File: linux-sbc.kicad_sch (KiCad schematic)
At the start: 9 parts, among them J101 Molex Mini-fit Jr

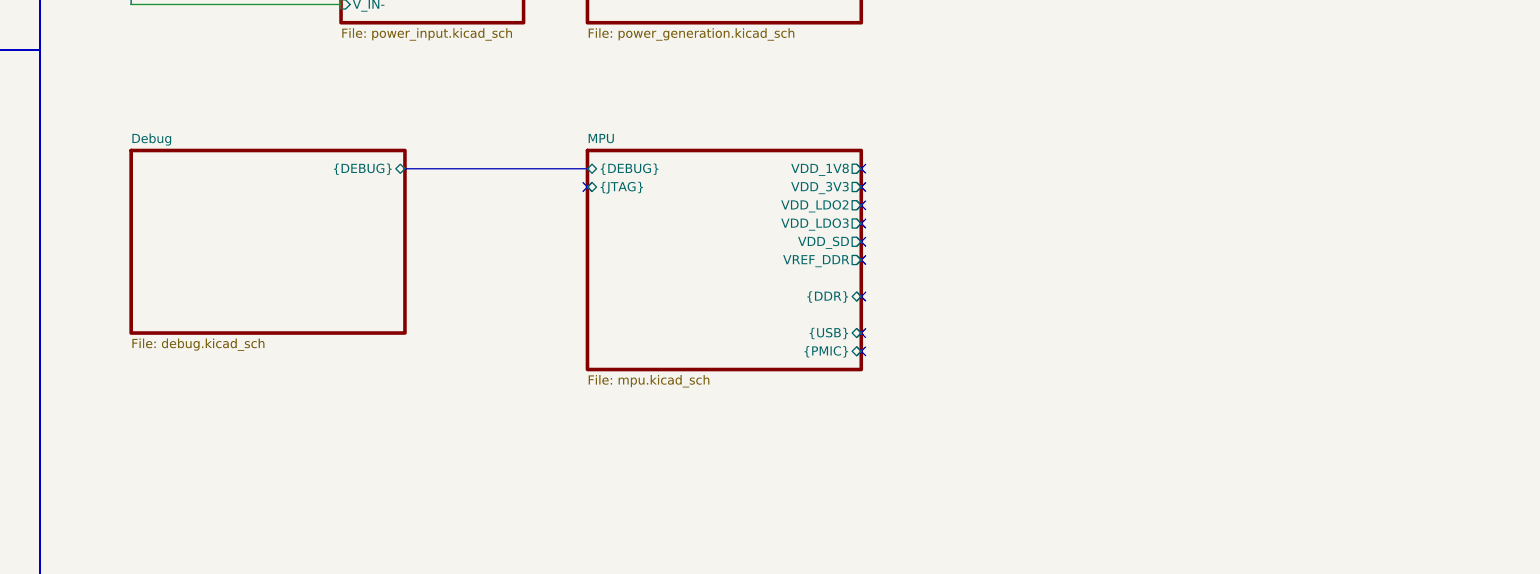
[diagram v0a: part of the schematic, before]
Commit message: Add a debug section
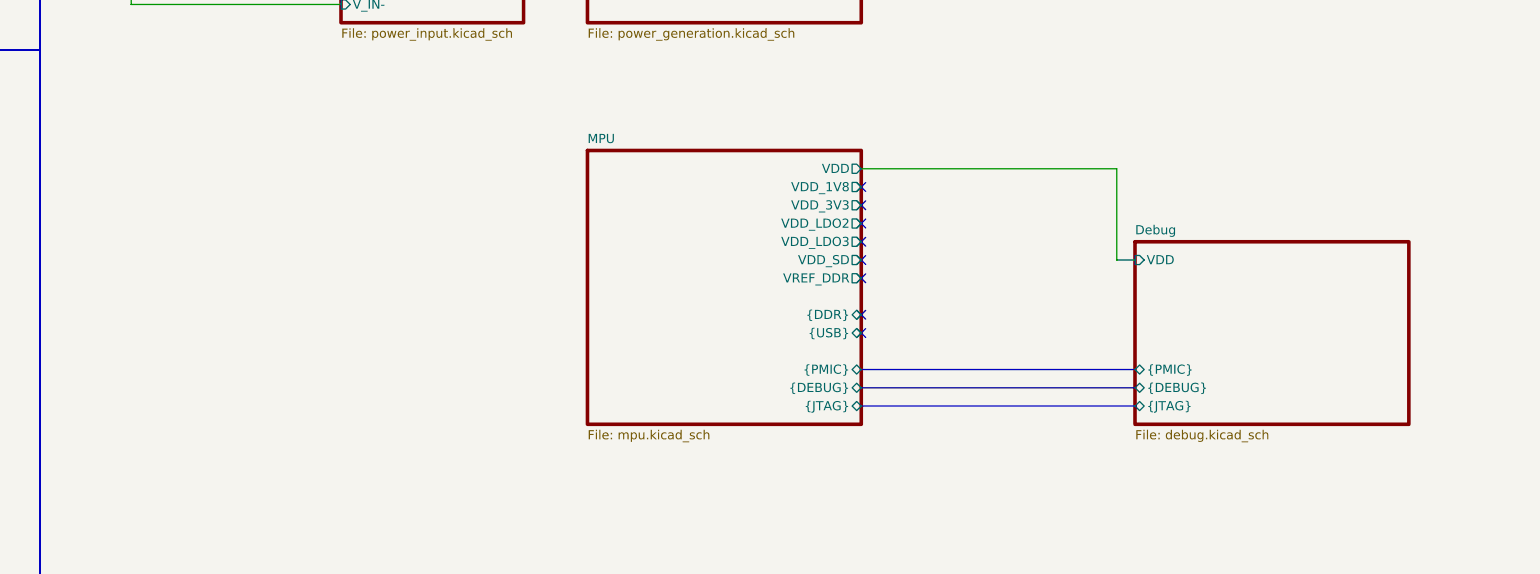
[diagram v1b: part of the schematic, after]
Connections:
- no-connect marks 10 -> 8
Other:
- sheet Debug ports: added VDD, {JTAG}, {PMIC}; removed none
- sheet MPU ports: added VDD; removed none
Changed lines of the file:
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@@
 			)
 			(justify left)
-			(href "#3")
+			(href "#4")
 		)
 	)
@@
 			)
 			(justify left)
-			(href "#3")
+			(href "#7")
 		)
 	)
@@
 			)
 			(justify left)
-			(href "#4")
+			(href "#6")
 		)
 	)
@@
 			)
 			(justify left)
-			(href "#4")
+			(href "#5")
 		)
 	)
@@
 	)
 	(no_connect
+		(at 254 139.7)
+	)
+	(no_connect
+		(at 254 144.78)
+	)
+	(no_connect
 		(at 254 137.16)
 	)
 	(no_connect
-		(at 215.9 132.08)
+		(at 254 149.86)
+	)
+	(no_connect
+		(at 254 132.08)
 	)
 	(no_connect
@@
 	)
 	(no_connect
+		(at 254 152.4)
+	)
+	(no_connect
 		(at 254 134.62)
 	)
-	(no_connect
-		(at 254 147.32)
-	)
-	(no_connect
-		(at 254 129.54)
-	)
-	(no_connect
-		(at 254 139.7)
-	)
-	(no_connect
-		(at 254 154.94)
-	)
-	(no_connect
-		(at 254 152.4)
-	)
-	(no_connect
-		(at 254 132.08)
-	)
 	(wire
 		(pts
@@
 		)
 	)
+	(bus
+		(pts
+			(xy 254 162.56) (xy 292.1 162.56)
+		)
+		(stroke
+			(width 0)
+			(type default)
+		)
+	)
 	(wire
 		(pts
@@
 	(wire
 		(pts
+			(xy 289.56 142.24) (xy 292.1 142.24)
+		)
+		(stroke
+			(width 0)
+			(type default)
+		)
+	)
+	(wire
+		(pts
 			(xy 167.64 88.9) (xy 167.64 91.44)
 		)
@@
 	(wire
 		(pts
+			(xy 289.56 129.54) (xy 289.56 142.24)
+		)
+		(stroke
+			(width 0)
+			(type default)
+		)
+	)
+	(wire
+		(pts
 			(xy 166.37 88.9) (xy 167.64 88.9)
 		)
@@
 		)
 	)
+	(bus
+		(pts
+			(xy 254 160.02) (xy 292.1 160.02)
+		)
+		(stroke
+			(width 0)
+			(type default)
+		)
+	)
+	(bus
+		(pts
+			(xy 254 157.48) (xy 292.1 157.48)
+		)
+		(stroke
+			(width 0)
+			(type default)
+		)
+	)
 	(wire
 		(pts
@@
 		)
 	)
-	(bus
-		(pts
-			(xy 190.5 129.54) (xy 215.9 129.54)
+	(wire
+		(pts
+			(xy 254 129.54) (xy 289.56 129.54)
 		)
 		(stroke
@@
 	(sheet
 		(at 215.9 127)
-		(size 38.1 30.48)
+		(size 38.1 38.1)
 		(exclude_from_sim no)
 		(in_bom yes)
@@
 		)
 		(property "Sheetfile" "mpu.kicad_sch"
-			(at 215.9 158.2384 0)
+			(at 215.9 165.8584 0)
 			(effects
 				(font
@@
 		)
 		(pin "{DDR}" bidirectional
-			(at 254 147.32 0)
+			(at 254 149.86 0)
 			(effects
 				(font
@@
 		)
 		(pin "{JTAG}" bidirectional
-			(at 215.9 132.08 180)
-			(effects
-				(font
-					(size 1.27 1.27)
-				)
-				(justify left)
+			(at 254 162.56 0)
+			(effects
+				(font
+					(size 1.27 1.27)
+				)
+				(justify right)
 			)
 		)
@@
 		)
 		(pin "VDD_1V8" output
+			(at 254 132.08 0)
+			(effects
+				(font
+					(size 1.27 1.27)
+				)
+				(justify right)
+			)
+		)
+		(pin "VDD_3V3" output
+			(at 254 134.62 0)
+			(effects
+				(font
+					(size 1.27 1.27)
+				)
+				(justify right)
+			)
+		)
+		(pin "VDD_LDO2" output
+			(at 254 137.16 0)
+			(effects
+				(font
+					(size 1.27 1.27)
+				)
+				(justify right)
+			)
+		)
+		(pin "VDD_LDO3" output
+			(at 254 139.7 0)
+			(effects
+				(font
+					(size 1.27 1.27)
+				)
+				(justify right)
+			)
+		)
+		(pin "VDD_SD" output
+			(at 254 142.24 0)
+			(effects
+				(font
+					(size 1.27 1.27)
+				)
+				(justify right)
+			)
+		)
+		(pin "VREF_DDR" output
+			(at 254 144.78 0)
+			(effects
+				(font
+					(size 1.27 1.27)
+				)
+				(justify right)
+			)
+		)
+		(pin "{PMIC}" bidirectional
+			(at 254 157.48 0)
+			(effects
+				(font
+					(size 1.27 1.27)
+				)
+				(justify right)
+			)
+		)
+		(pin "{DEBUG}" bidirectional
+			(at 254 160.02 0)
+			(effects
+				(font
+					(size 1.27 1.27)
+				)
+				(justify right)
+			)
+		)
+		(pin "VDD" output
 			(at 254 129.54 0)
 			(effects
@@
 				)
 				(justify right)
-			)
-		)
-		(pin "VDD_3V3" output
-			(at 254 132.08 0)
-			(effects
-				(font
-					(size 1.27 1.27)
-				)
-				(justify right)
-			)
-		)
-		(pin "VDD_LDO2" output
-			(at 254 134.62 0)
-			(effects
-				(font
-					(size 1.27 1.27)
-				)
-				(justify right)
-			)
-		)
-		(pin "VDD_LDO3" output
-			(at 254 137.16 0)
-			(effects
-				(font
-					(size 1.27 1.27)
-				)
-				(justify right)
-			)
-		)
-		(pin "VDD_SD" output
-			(at 254 139.7 0)
-			(effects
-				(font
-					(size 1.27 1.27)
-				)
-				(justify right)
-			)
-		)
-		(pin "VREF_DDR" output
-			(at 254 142.24 0)
-			(effects
-				(font
-					(size 1.27 1.27)
-				)
-				(justify right)
-			)
-		)
-		(pin "{PMIC}" bidirectional
-			(at 254 154.94 0)
-			(effects
-				(font
-					(size 1.27 1.27)
-				)
-				(justify right)
-			)
-		)
-		(pin "{DEBUG}" bidirectional
-			(at 215.9 129.54 180)
-			(effects
-				(font
-					(size 1.27 1.27)
-				)
-				(justify left)
 			)
 		)
@@
 	)
 	(sheet
-		(at 152.4 127)
+		(at 292.1 139.7)
 		(size 38.1 25.4)
 		(exclude_from_sim no)
@@
 		)
 		(property "Sheetname" "Debug"
-			(at 152.4 126.1146 0)
+			(at 292.1 138.8146 0)
 			(effects
 				(font
@@
 		)
 		(property "Sheetfile" "debug.kicad_sch"
-			(at 152.4 153.1584 0)
+			(at 292.1 165.8584 0)
 			(effects
 				(font
@@
 		)
 		(pin "{DEBUG}" bidirectional
-			(at 190.5 129.54 0)
-			(effects
-				(font
-					(size 1.27 1.27)
-				)
-				(justify right)
-			)
-		)
+			(at 292.1 160.02 180)
+			(effects
+				(font
+					(size 1.27 1.27)
+				)
+				(justify left)
+			)
+		)
+		(pin "VDD" input
+			(at 292.1 142.24 180)
+			(effects
+				(font
+					(size 1.27 1.27)
+				)
+				(justify left)
+			)
+		)
+		(pin "{JTAG}" bidirectional
+			(at 292.1 162.56 180)
+			(effects
+				(font
+					(size 1.27 1.27)
+				)
+				(justify left)
+			)
+		)
+		(pin "{PMIC}" bidirectional
+			(at 292.1 157.48 180)
+			(effects
+				(font
+					(size 1.27 1.27)
+				)
+				(justify left)
+			)
+		)
